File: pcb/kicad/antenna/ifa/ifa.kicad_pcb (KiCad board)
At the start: 2 copper layers, 29.6 x 24.1 mm, 1 part, among them P1 CONN_01X02

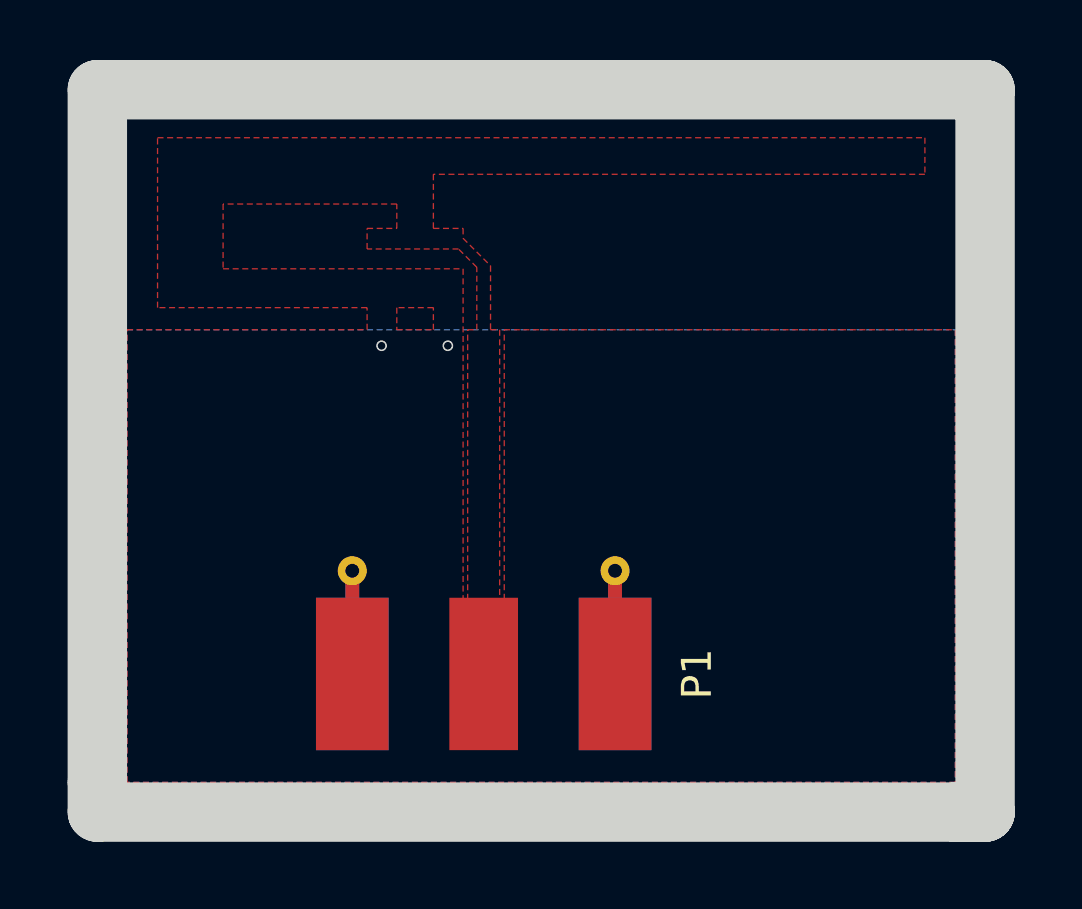
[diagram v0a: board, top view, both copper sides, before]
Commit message: Cleanup vias on layout
Layout is essentially complete, but concerned about the lack of physical
connection between SMA signal and antenna feedline. Further attempts,
especially fill, to fix this introduced more problems with the rest of
the layout.
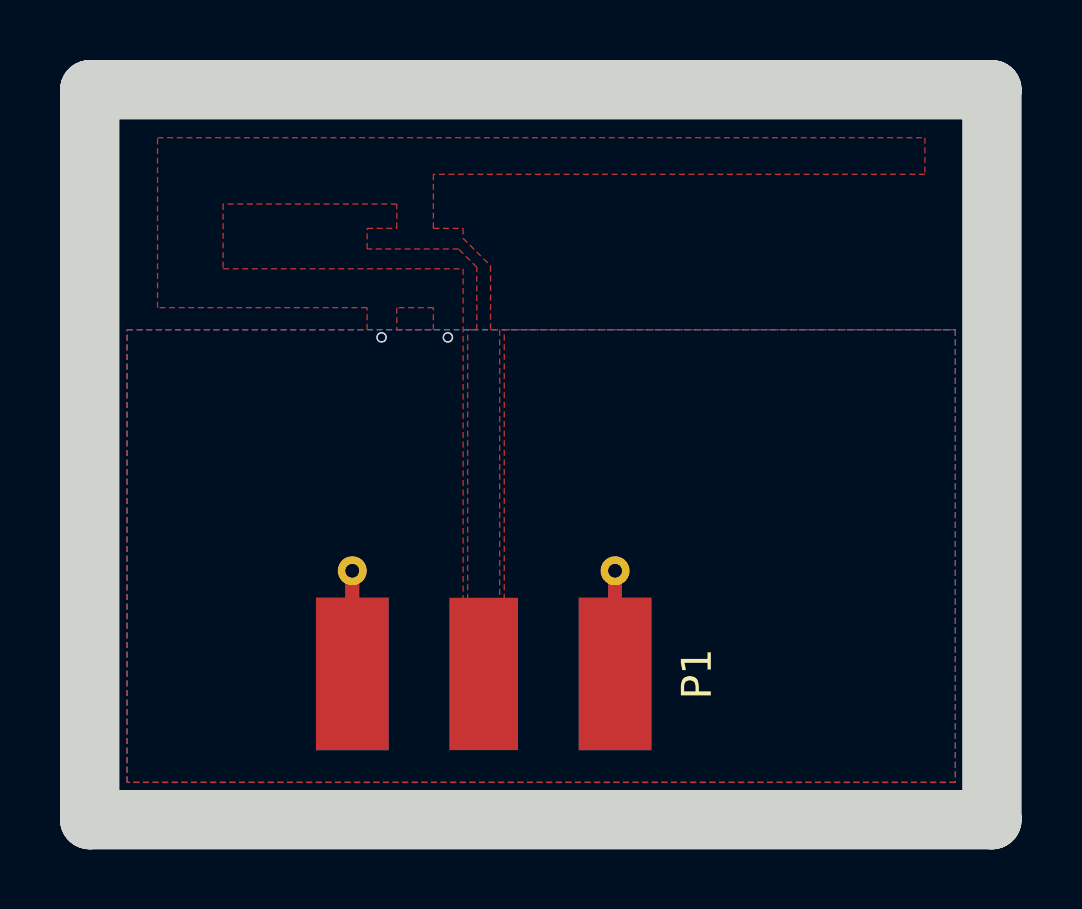
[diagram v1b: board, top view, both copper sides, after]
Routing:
- net GND: vias 0 -> 2
- net (no net): vias 2 -> 0
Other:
- board size 29.6 x 24.1 mm -> 30.1 x 24.3 mm
- net class Default: trace_width 0.127 -> 0.254
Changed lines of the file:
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@@
   (general
     (links 10)
-    (no_connects 4)
-    (area 107.238799 56.438799 138.811001 82.499201)
+    (no_connects 3)
+    (area 128.193799 76.149199 272.295714 194.39)
     (thickness 1.6)
-    (drawings 10)
+    (drawings 11)
     (tracks 2)
     (zones 0)
@@
   (setup
     (last_trace_width 0.254)
-    (user_trace_width 0.254)
     (trace_clearance 0.254)
     (zone_clearance 0.508)
-    (zone_45_only no)
+    (zone_45_only yes)
     (trace_min 0.127)
     (segment_width 0.2)
@@
     (via_min_size 0.254)
     (via_min_drill 0.254)
+    (user_via 1.524 1.27)
+    (user_via 1.778 1.016)
+    (user_via 1.778 1.27)
+    (user_via 1.778 1.524)
+    (user_via 2.032 1.27)
     (uvia_size 0.3)
     (uvia_drill 0.1)
@@
     (mod_text_width 0.15)
     (pad_size 5.08 2.29)
-    (pad_drill 0)
+    (pad_drill 0.6)
     (pad_to_mask_clearance 0.2)
-    (aux_axis_origin 10.16 10.16)
-    (visible_elements FFFFFF7F)
+    (aux_axis_origin 130.429 100.2284)
+    (grid_origin 130.429 100.2284)
+    (visible_elements 7FFFFFFF)
     (pcbplotparams
-      (layerselection 0x010f0_80000001)
+      (layerselection 0x030f0_80000001)
       (usegerberextensions false)
       (excludeedgelayer true)
@@
   (net_class Default "This is the default net class."
     (clearance 0.254)
-    (trace_width 0.127)
+    (trace_width 0.254)
     (via_dia 0.3556)
     (via_drill 0.254)
@@
       (net 1 GND))
   )
-  (gr_line (start 159.0294 101.219) (end 159.0294 77.1398) (angle 90) (layer Edge.Cuts) (width 1.9812))
-  (gr_line (start 158.0388 101.219) (end 159.0294 101.219) (angle 90) (layer Edge.Cuts) (width 1.9812))
-  (gr_line (start 129.4384 101.219) (end 159.0294 101.219) (angle 90) (layer Edge.Cuts) (width 1.9812))
-  (gr_line (start 129.4384 100.2284) (end 129.4384 101.219) (angle 90) (layer Edge.Cuts) (width 1.9812))
-  (gr_line (start 129.4384 77.1398) (end 129.4384 100.2284) (angle 90) (layer Edge.Cuts) (width 1.9812))
-  (gr_line (start 159.004 77.1398) (end 159.0294 77.1398) (angle 90) (layer Edge.Cuts) (width 1.9812))
-  (gr_line (start 129.4384 77.1398) (end 159.004 77.1398) (angle 90) (layer Edge.Cuts) (width 1.9812))
+  (gr_line (start 158.0388 78.1304) (end 130.429 78.1304) (layer Margin) (width 0.2))
+  (gr_line (start 158.0388 100.2284) (end 158.0388 78.1304) (layer Margin) (width 0.2))
+  (gr_line (start 130.429 100.2284) (end 158.0388 100.2284) (layer Margin) (width 0.2))
+  (gr_line (start 130.429 78.1304) (end 130.429 100.2284) (layer Margin) (width 0.2))
+  (gr_line (start 129.1844 77.1398) (end 129.1844 101.473) (angle 90) (layer Edge.Cuts) (width 1.9812))
+  (gr_line (start 159.258 101.473) (end 159.258 77.1398) (angle 90) (layer Edge.Cuts) (width 1.9812))
+  (gr_line (start 129.1844 101.473) (end 159.258 101.473) (angle 90) (layer Edge.Cuts) (width 1.9812))
+  (gr_line (start 159.258 77.1398) (end 129.1844 77.1398) (angle 90) (layer Edge.Cuts) (width 1.9812))
   (gr_text 0.1 (at 270.51 193.04) (layer Cmts.User)
     (effects (font (size 1.5 1.5) (thickness 0.3)))
@@
     (effects (font (size 1.5 1.5) (thickness 0.3)))
   )
-  (via (at 138.9126 85.6742) (size 0.3556) (drill 0.254) (layers F.Cu B.Cu) (net 0))
-  (via (at 141.1224 85.6742) (size 0.3556) (drill 0.254) (layers F.Cu B.Cu) (net 0))
+  (via (at 138.9126 85.3948) (size 0.3556) (drill 0.254) (layers F.Cu B.Cu) (net 1))
+  (via (at 141.1224 85.3948) (size 0.3556) (drill 0.254) (layers F.Cu B.Cu) (net 1))
   (zone (net 1) (net_name GND) (layer F.Cu) (hatch edge 0.508)
     (connect_pads (clearance 0.254))
